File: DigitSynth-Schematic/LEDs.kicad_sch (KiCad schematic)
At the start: 4 parts, among them J5 Conn_01x05_Pin, J6 Conn_01x02_Pin

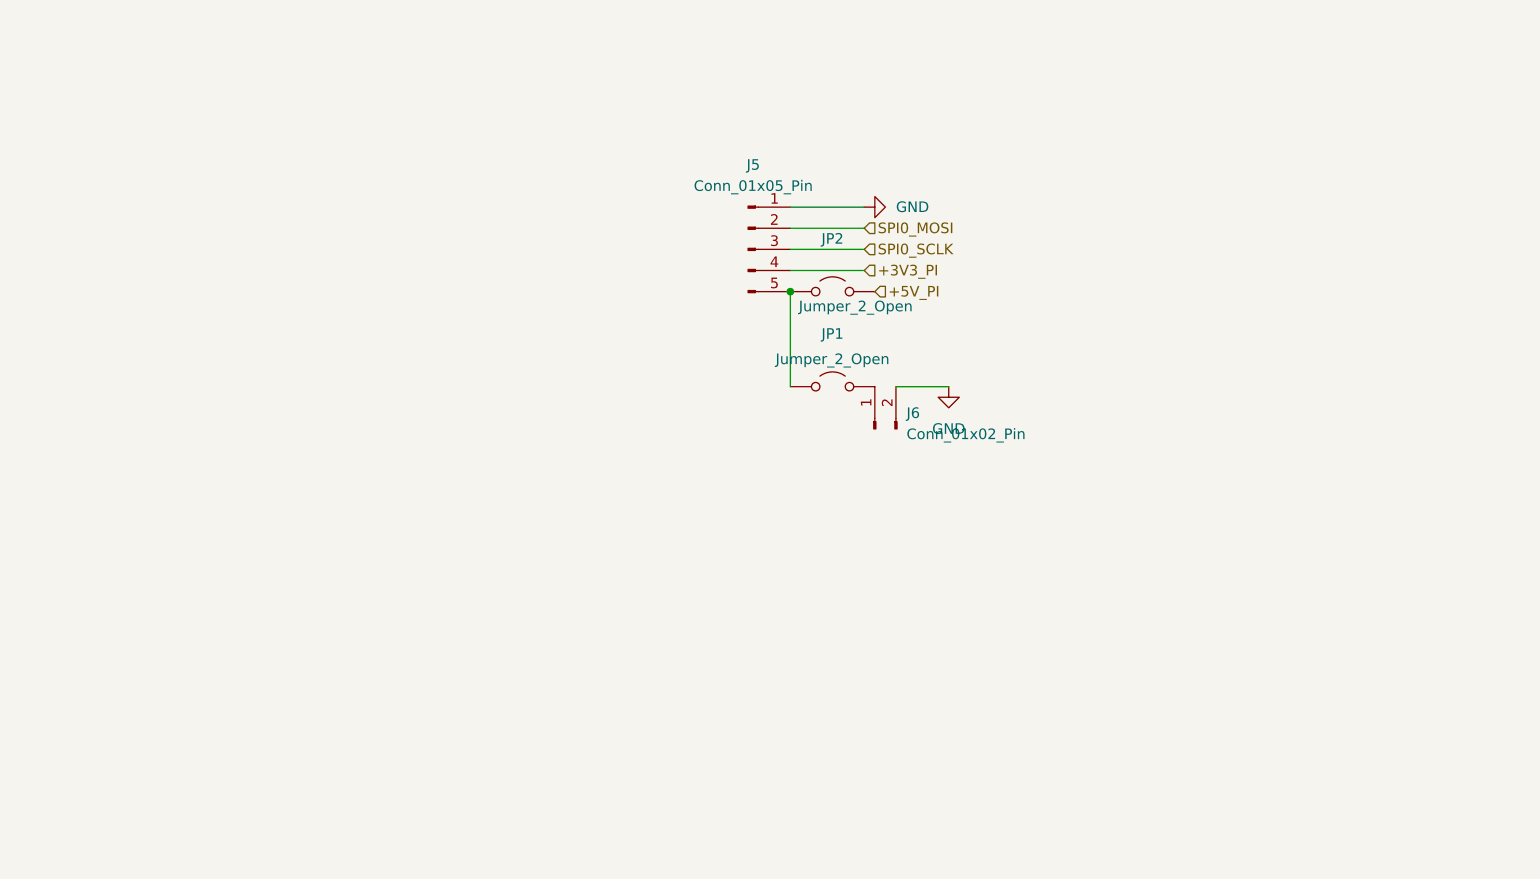
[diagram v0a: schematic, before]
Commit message: KiCad PCB fully routed
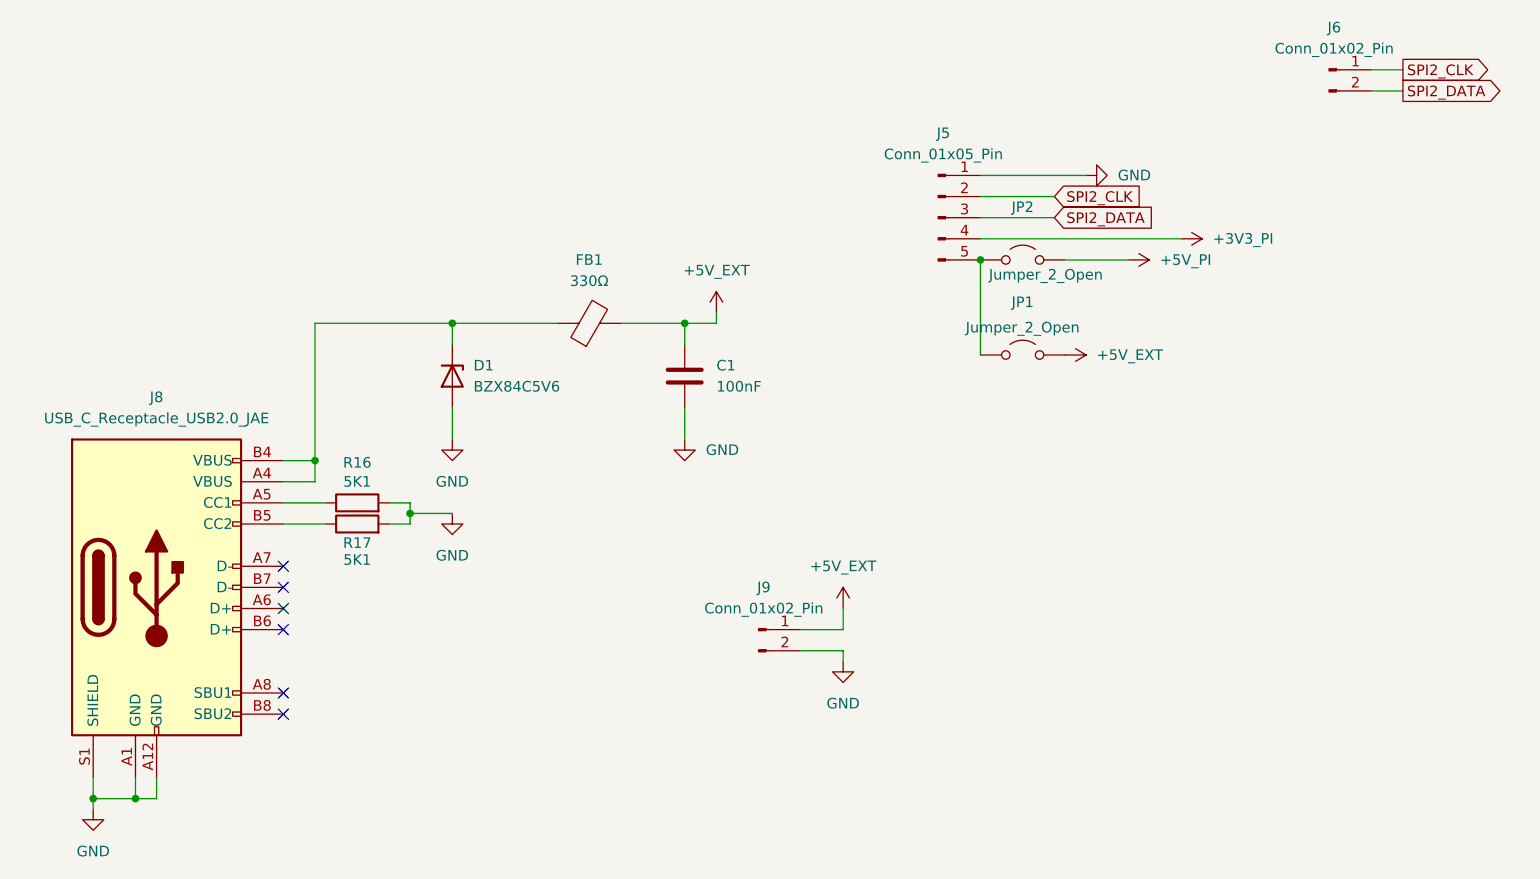
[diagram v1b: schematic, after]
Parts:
- added C1: 100nF, Capacitor_SMD:C_0603_1608Metric, symbol Device:C
- added D1: BZX84C5V6, Package_TO_SOT_SMD:SOT-23, symbol Diode:BZX84Cxx
- added FB1: 330Ω, Inductor_SMD:L_0603_1608Metric, symbol Device:FerriteBead
- added J8: USB_C_Receptacle_USB2.0_JAE, footprints:JAE_DX07S016JA1R1500, symbol CUSTOMCONN:USB_C_Receptacle_USB2.0_JAE
- added J9: Conn_01x02_Pin, Connector_Molex:Molex_KK-254_AE-6410-02A_1x02_P2.54mm_Vertical, symbol Connector:Conn_01x02_Pin
- added R16, R17: 5K1, Resistor_SMD:R_0603_1608Metric, symbol Device:R
- J5: footprint (none) -> Connector_Molex:Molex_KK-254_AE-6410-05A_1x05_P2.54mm_Vertical
- J6: footprint (none) -> Connector_Molex:Molex_KK-254_AE-6410-02A_1x02_P2.54mm_Vertical
- JP1, JP2: footprint (none) -> Jumper:SolderJumper-2_P1.3mm_Open_RoundedPad1.0x1.5mm
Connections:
- net GND: now also C1.2, D1.1 (A), J8.A1 (GND), J8.A12 (GND), J8.S1 (SHIELD), J9.2 (Pin_2), R16.2, R17.2; no longer J6.2 (Pin_2)
- net +5V_EXT: now reaches JP1.2 (B)
- net +5V_EXT: now also C1.1, FB1.2, J9.1 (Pin_1); no longer J6.1 (Pin_1)
- net SPI0_MOSI renamed SPI2_CLK
- net SPI2_CLK: now also J6.1 (Pin_1)
- net SPI0_SCLK renamed SPI2_DATA
- net SPI2_DATA: now also J6.2 (Pin_2)
- new net: D1.3 (K), FB1.1, J8.A4 (VBUS), J8.B4 (VBUS)
- new net: J8.B5 (CC2), R17.1
- new net: J8.A5 (CC1), R16.1
- no-connect marks 0 -> 6
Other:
- moved on the sheet: J5, JP1, JP2
